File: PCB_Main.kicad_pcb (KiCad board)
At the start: 2 copper layers, 118 x 53.3 mm, 33 parts, among them J1 Power, J2 PWM, J3 Analog, J4 PWM, J5 Analog, J6 Communication, M78AR05-1 M78AR05, M78AR05-2 M78AR05, M78AR05-3 M78AR05, U1 MOUDLE-SEEEDUINO-XIAO, Y1 16MHｚ

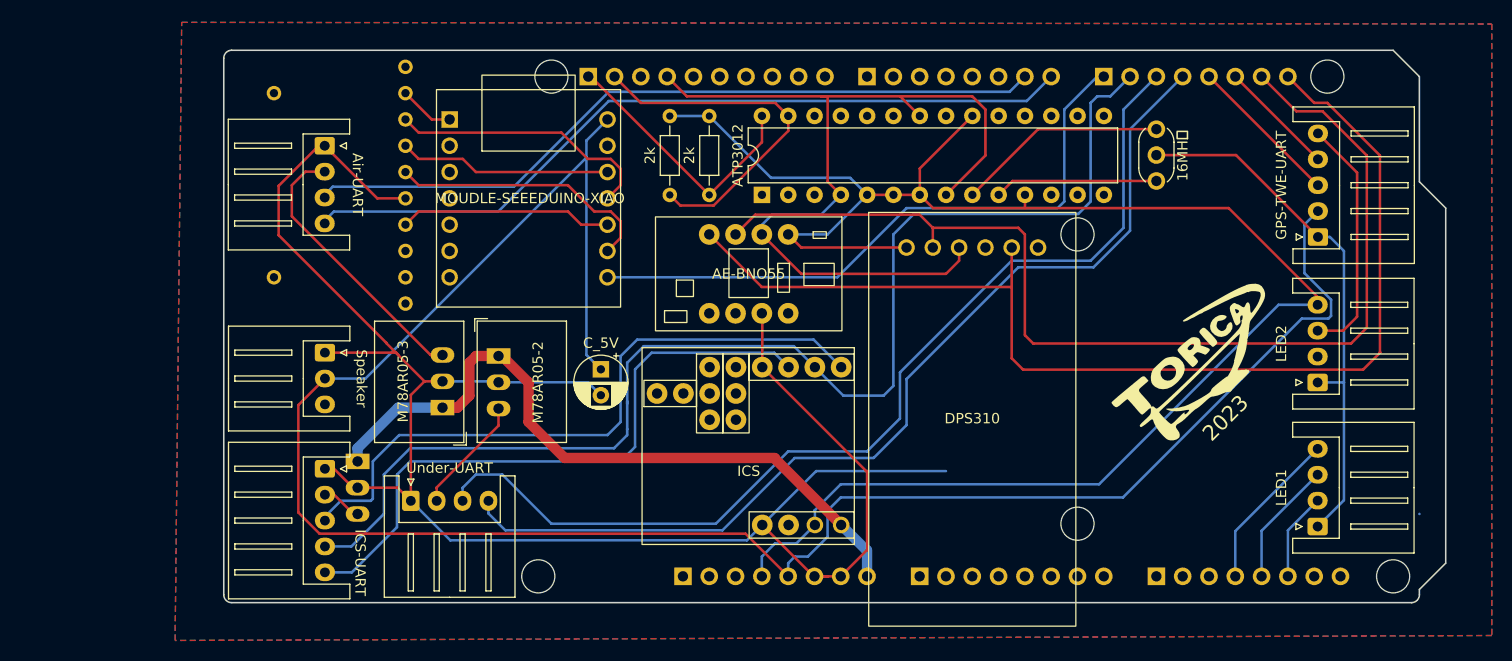
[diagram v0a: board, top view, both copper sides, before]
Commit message: update
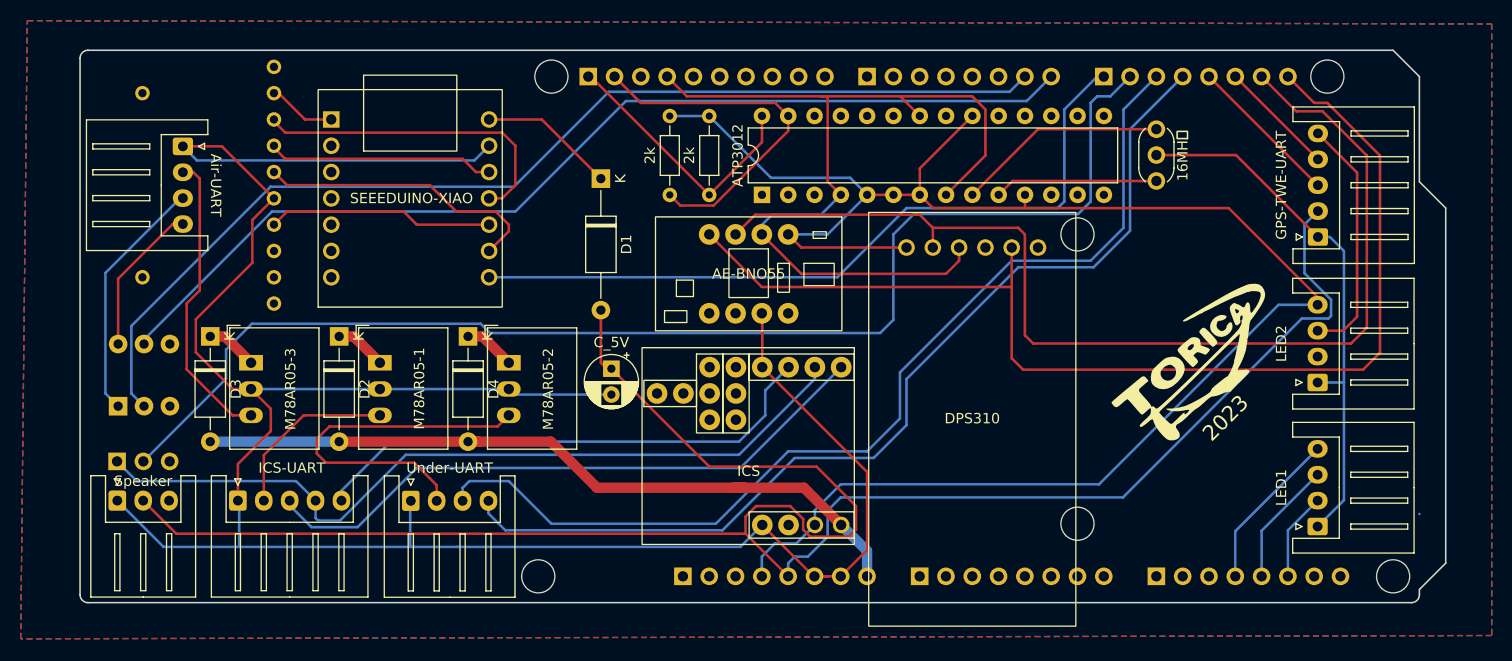
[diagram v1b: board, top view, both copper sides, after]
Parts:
- added D1: D, Diode_THT:D_A-405_P12.70mm_Horizontal, F.Cu at (120.0, 59.1)
- added D2: D, Diode_THT:D_A-405_P10.16mm_Horizontal, F.Cu at (94.7, 74.3)
- added D3: D, Diode_THT:D_A-405_P10.16mm_Horizontal, F.Cu at (82.3, 74.3)
- added D4: D, Diode_THT:D_A-405_P10.16mm_Horizontal, F.Cu at (107.2, 74.3)
- added ICS-SW1: SW_DPDT_x2, Connector_PinHeader_2.54mm:PinHeader_1x03_P2.54mm_Vertical, B.Cu at (73.3, 86.4)
- added Serial-SW1: SW_DPDT_x2, Button_Switch_THT:SW_Push_2P2T_Toggle_CK_PVA2OAH5xxxxxxV2, B.Cu at (73.4, 81.0)
- M78AR05-1: moved to F.Cu
- U1: value MOUDLE-SEEEDUINO-XIAO -> SEEEDUINO-XIAO
- moved Speaker1 24.6 mm to (73.3, 90.1), turned to 0 degrees
- moved M78AR05-3 19.0 mm to (86.2, 76.8), turned to -90 degrees
- moved Air-UART1 13.7 mm to (79.7, 55.9)
- moved AE-MICRO-SD-DIP1 12.7 mm to (89.7, 59.7)
- moved U1 11.4 mm to (101.6, 61.0)
- moved M78AR05-1 9.77 mm to (98.7, 76.8)
- moved ICS-UART1 8.95 mm to (85.0, 90.1), turned to 0 degrees
- moved M78AR05-2 1.19 mm to (111.1, 76.8)
- moved C1 1.02 mm to (121.0, 77.4)
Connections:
- J4 pad 7: DTAR -> /TX0/1
- J4 pad 8: DRAT -> /RX0/0
- J6 pad 2: IRXT -> /RX3/15
- M78AR05-1 pad 1: VCC -> Net-(M78AR05-1-Pad1)
- M78AR05-2 pad 1: VCC -> Net-(M78AR05-2-Pad1)
- M78AR05-3 pad 1: VCC -> Net-(M78AR05-3-Pad1)
- U1 pad 14: 5V -> Net-(U1-Pad14)
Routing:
- net /RX3/15: track 0.00 -> 123.5 mm
- net /TX0/1: track 0.00 -> 104.5 mm
- net /RX0/0: track 0.00 -> 98.6 mm
- net DRAT: track 76.2 -> 14.7 mm
- net DTAR: track 72.6 -> 23.8 mm
- net GND: track 324.0 -> 369.4 mm
- net IRXT: track 121.8 -> 77.5 mm
- net Net-(M78AR05-2-Pad3): track 11.4 -> 35.2 mm
- net Net-(ICS-UART1-Pad2): track 3.94 -> 17.6 mm
- net Net-(U1-Pad14): track 0.00 -> 13.2 mm
- net DTSR: track 61.2 -> 72.6 mm
- net EN: track 61.9 -> 50.5 mm
- net 5V: track 200.0 -> 194.7 mm
- net SD-MOSI: track 26.1 -> 31.3 mm
- net Net-(M78AR05-3-Pad1): track 0.00 -> 4.99 mm
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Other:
- board size 118 x 53.3 mm -> 131.9 x 53.3 mm

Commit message: jlcpcb
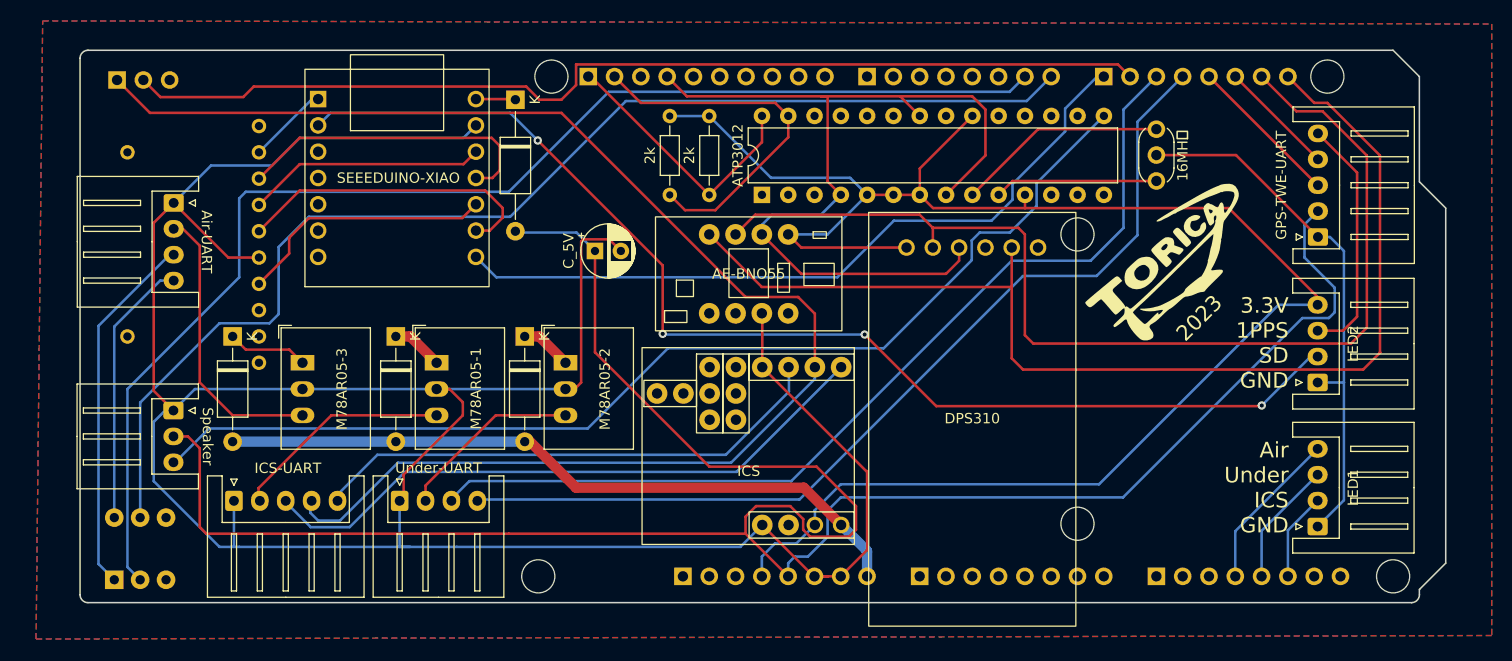
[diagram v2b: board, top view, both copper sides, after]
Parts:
- moved ICS-SW1 36.8 mm to (73.3, 49.5)
- moved Serial-SW1 16.8 mm to (73.0, 97.8)
- moved C1 11.5 mm to (119.4, 66.0), turned to 0 degrees
- moved D1 11.2 mm to (111.8, 51.4)
- moved Speaker1 10.3 mm to (78.7, 81.4), turned to -90 degrees
- moved G*** 9.98 mm to (175.3, 67.4)
- moved AE-MICRO-SD-DIP1 5.90 mm to (88.3, 65.4)
- moved Air-UART1 5.53 mm to (78.8, 61.4)
- moved D2 5.47 mm to (100.2, 74.3)
- moved D4 5.47 mm to (112.7, 74.3)
- moved M78AR05-1 5.47 mm to (104.2, 76.8)
- moved M78AR05-2 5.47 mm to (116.6, 76.8)
- moved M78AR05-3 4.97 mm to (91.2, 76.8)
- moved U1 2.34 mm to (100.3, 59.0)
- moved D3 2.16 mm to (84.5, 74.3)
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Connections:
- ATP3012 pad 15: unconnected-(ATP3012-Pad15) -> Net-(ATP3012-Pad15)
- LED2 pad 2: unconnected-(LED2-Pad2) -> L_SD
- Speaker1 pad 3: unconnected-(Speaker1-Pad3) -> Net-(ATP3012-Pad15)
- U1 pad 2: unconnected-(U1-Pad2) -> L_SD
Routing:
- net L_SD: track 0.00 -> 114.8 mm, vias 0 -> 4
- net Net-(ATP3012-Pad15): track 0.00 -> 106.1 mm
- net IRXT: track 77.5 -> 139.4 mm
- net GND: track 369.4 -> 398.8 mm
- net /RX3/15: track 123.5 -> 100.0 mm
- net 5V: track 194.7 -> 213.3 mm
- net /TX0/1: track 104.5 -> 122.6 mm
- net Net-(M78AR05-2-Pad3): track 35.2 -> 17.8 mm
- net /RX0/0: track 98.6 -> 115.9 mm
- net DTAR: track 23.8 -> 35.3 mm
- net DRAT: track 14.7 -> 26.0 mm
- net Net-(D1-Pad1): track 13.2 -> 3.84 mm
- net DTUR: track 97.4 -> 91.9 mm
- net VCC: track 72.4 -> 68.1 mm
- net DRUT: track 95.4 -> 91.5 mm
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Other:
- board text added: "3.3V 1PPS SD GND"
- board text added: "Air Under ICS GND"
- board text removed: "ICSP"
